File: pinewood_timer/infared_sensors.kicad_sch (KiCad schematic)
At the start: 0 parts

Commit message: worked on schematic more
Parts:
- added D1, D2, D3, D4: LED, LED_THT:LED_D5.0mm, symbol Device:LED
- added PT1, PT2, PT3, PT4: ~, LED_THT:LED_D5.0mm, symbol 2N4403:PT204-6B
- added R33, R36, R38, R40: 56KΩ, symbol Device:R_Small_US
- added R34, R35, R37, R39: 220Ω, symbol Device:R_Small_US
- added R41, R42, R43, R44: 1KΩ, symbol Device:R_Small_US
- added RV1: 10k pot, symbol Device:R_Potentiometer_US
- added U10: LM339N, N14, symbol LM339:LM339N
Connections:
- new net: D4.2 (A), R39.2
- new net: D2.2 (A), R35.2
- new net: D3.2 (A), R37.2
- new net: D1.2 (A), R34.2
- new net +3.3V: PT1.1 (+), PT2.1 (+), PT3.1 (+), PT4.1 (+), R34.1, R35.1, R37.1, R39.1, R41.1, R42.1, R43.1, R44.1
- new net +5V: RV1.1, U10.3 (VCC)
- new net GND: D1.1 (K), D2.1 (K), D3.1 (K), D4.1 (K), R33.2, R36.2, R38.2, R40.2, RV1.3, U10.12 (GND)
- new net V_OUT1: R41.2, U10.1 (1OUT)
- new net V_OUT2: R42.2, U10.2 (2OUT)
- new net V_OUT3: R43.2, U10.14 (OUT3)
- new net V_OUT4: R44.2, U10.13 (OUT4)
- new net V_PT1: PT1.2 (-), R33.1, U10.7 (1IN+)
- new net V_PT2: PT2.2 (-), R36.1, U10.5 (2IN+)
- new net V_PT3: PT3.2 (-), R38.1, U10.9 (3IN+)
- new net V_PT4: PT4.2 (-), R40.1, U10.11 (4IN+)
- new net pot: RV1.2, U10.10 (4IN-), U10.4 (2IN-), U10.6 (1IN-), U10.8 (3IN-)
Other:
- note added: "this wont be a pot forever, it is jsut to adjust for the distance. afterwards, the resistor value will be taken and the pot will be replaced"
- title: (none) -> IR SENSORS

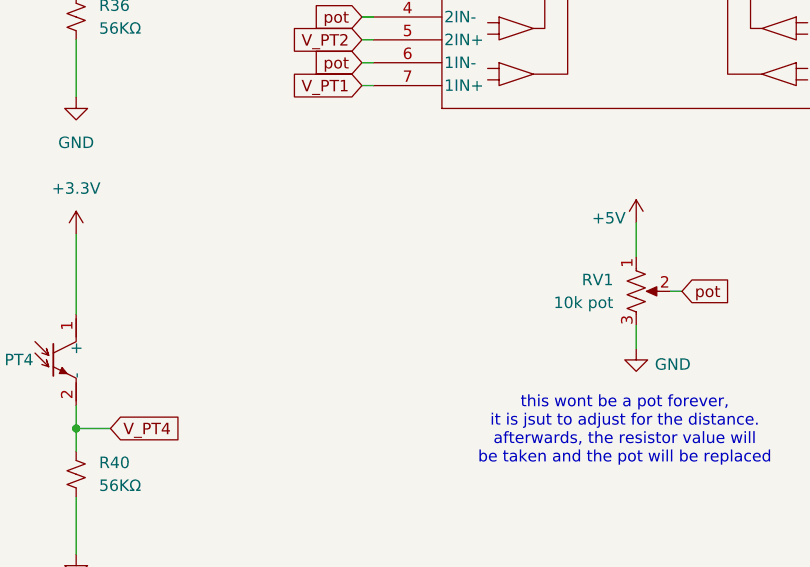
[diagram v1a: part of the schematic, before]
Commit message: added pins
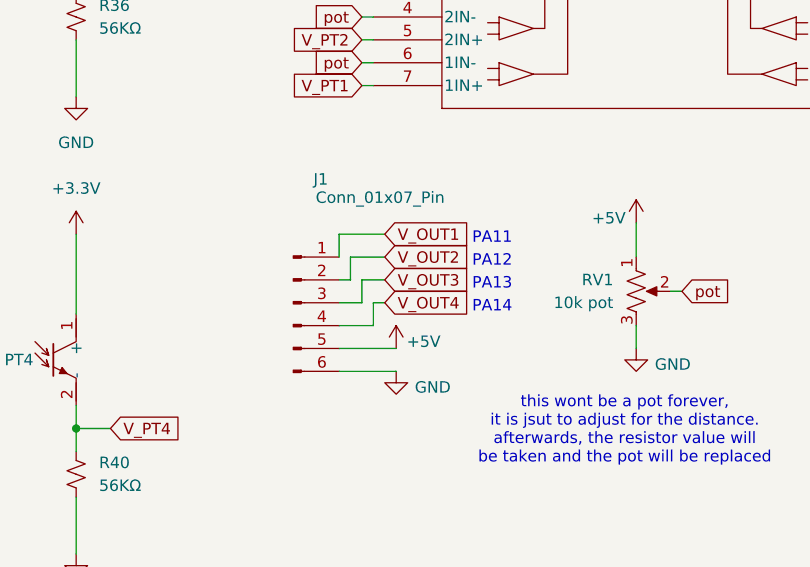
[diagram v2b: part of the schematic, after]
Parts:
- added J1: Conn_01x07_Pin, symbol Connector:Conn_01x06_Pin
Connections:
- net +5V: now also J1.5 (Pin_5)
- net GND: now also J1.6 (Pin_6)
- net V_OUT1: now also J1.1 (Pin_1)
- net V_OUT2: now also J1.2 (Pin_2)
- net V_OUT3: now also J1.3 (Pin_3)
- net V_OUT4: now also J1.4 (Pin_4)
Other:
- note added: "PA11"
- note added: "PA12"
- note added: "PA13"
- note added: "PA14"
